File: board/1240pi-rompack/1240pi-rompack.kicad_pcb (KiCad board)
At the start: 4 copper layers, 73.7 x 50.8 mm, 5 parts, among them J1 HDMI_A, J2 HDMI_A, P1 CardEdge_ROMPACK

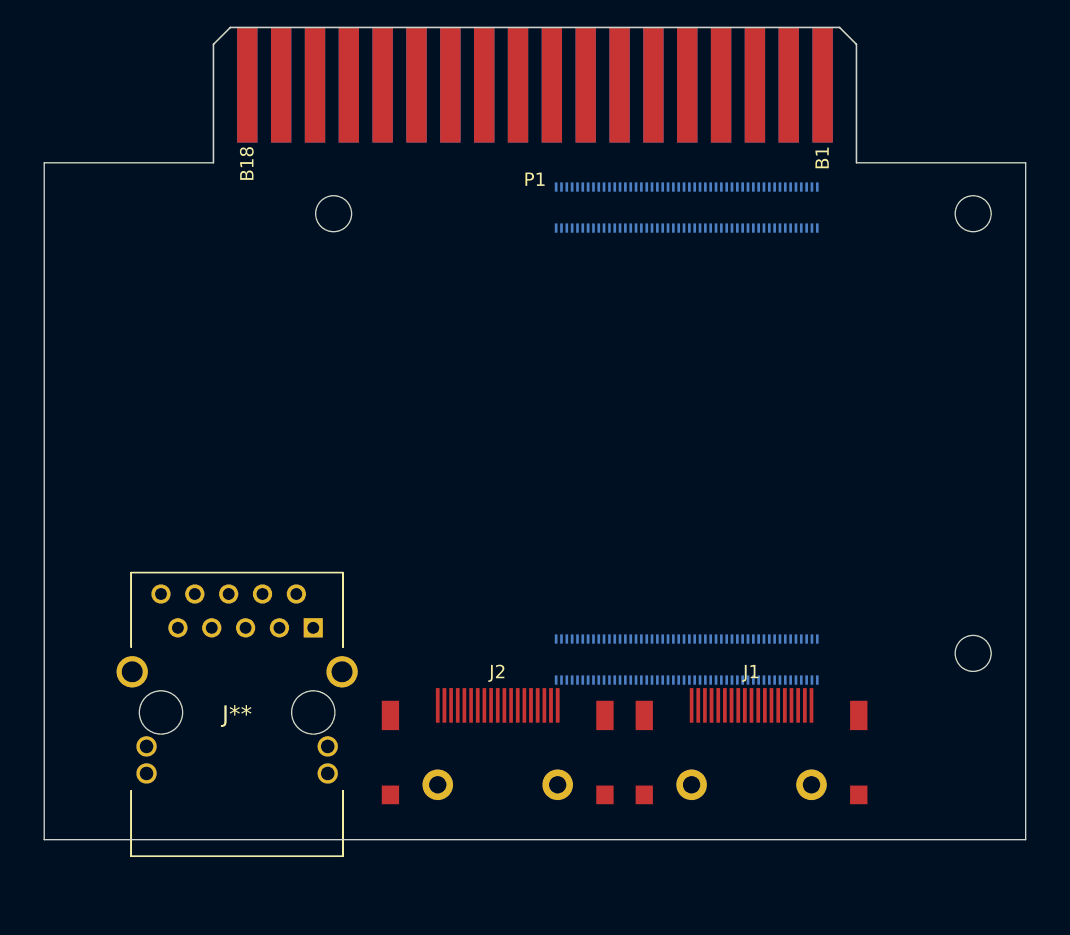
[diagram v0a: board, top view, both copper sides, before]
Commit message: Add more stuff to rompack board.
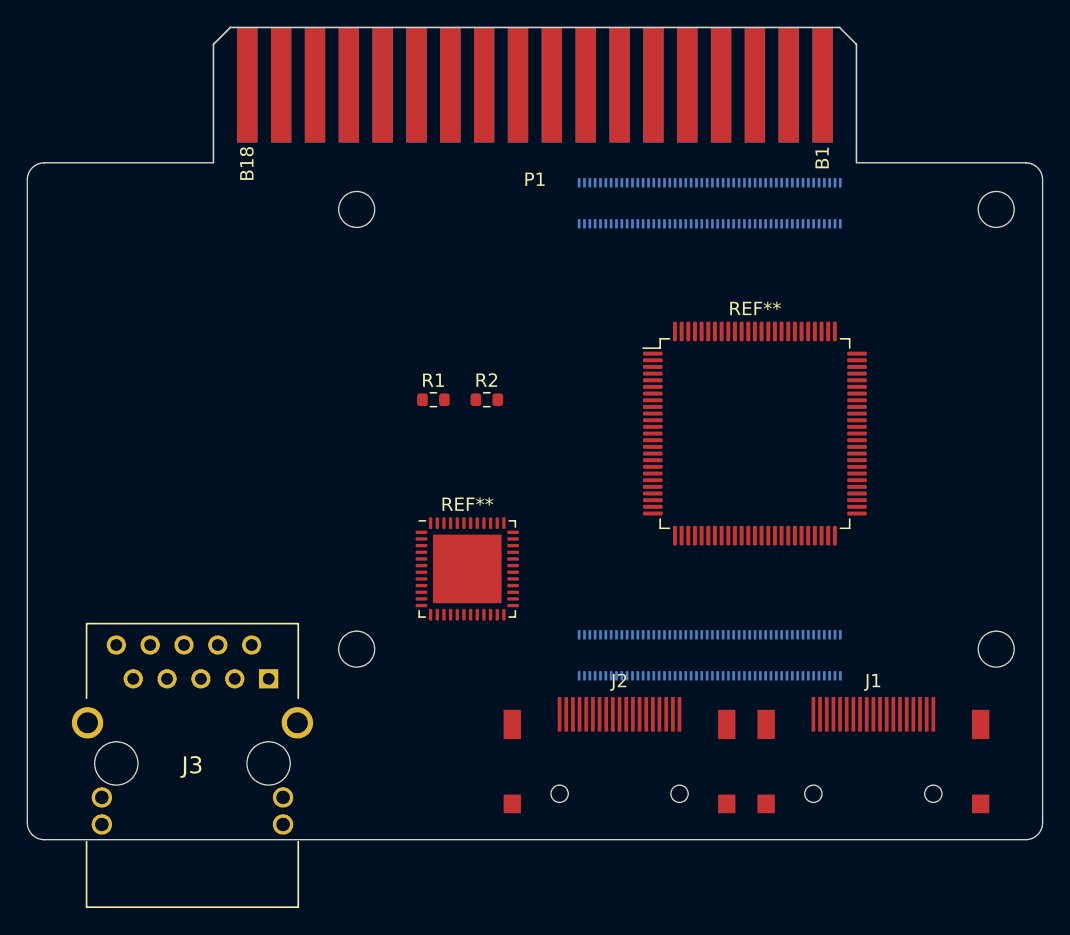
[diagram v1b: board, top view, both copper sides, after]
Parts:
- added R1: 470R, Resistor_SMD:R_0603_1608Metric, F.Cu at (144.8, 81.3)
- added R2: 470R, Resistor_SMD:R_0603_1608Metric, F.Cu at (148.8, 81.3)
- added REF**: QFN-48-1EP_7x7mm_P0.5mm_EP5.15x5.15mm, Package_DFN_QFN:QFN-48-1EP_7x7mm_P0.5mm_EP5.15x5.15mm, F.Cu at (147.3, 94.0)
- added REF**: VQFP-100_14x14mm_P0.5mm, Package_QFP:VQFP-100_14x14mm_P0.5mm, F.Cu at (168.9, 83.8)
- moved J1 9.17 mm to (177.8, 104.9)
- moved J2 9.17 mm to (158.8, 104.9)
- moved J3 5.09 mm to (132.4, 102.2)
- moved A1 1.76 mm to (187.0, 67.0)
- renumbered J** to J3
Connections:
- A1 pad 10: unconnected-(A1-Pad10) -> Net-(A1-Pad10)
- A1 pad 11: unconnected-(A1-Pad11) -> Net-(A1-Pad11)
- A1 pad 12: unconnected-(A1-Pad12) -> Net-(A1-Pad12)
- A1 pad 143: unconnected-(A1-Pad143) -> /HDMI/HDMI_OUT_HPD
- A1 pad 145: unconnected-(A1-Pad145) -> /HDMI/HDMI_OUT_SDA
- A1 pad 146: unconnected-(A1-Pad146) -> /HDMI/HDMI_OUT_D2_P
- A1 pad 147: unconnected-(A1-Pad147) -> /HDMI/HDMI_OUT_SCL
- A1 pad 148: unconnected-(A1-Pad148) -> /HDMI/HDMI_OUT_D2_N
- A1 pad 149: unconnected-(A1-Pad149) -> /HDMI/HDMI_OUT_CEC
- A1 pad 152: unconnected-(A1-Pad152) -> /HDMI/HDMI_OUT_D1_P
- A1 pad 154: unconnected-(A1-Pad154) -> /HDMI/HDMI_OUT_D1_N
- A1 pad 158: unconnected-(A1-Pad158) -> /HDMI/HDMI_OUT_D0_P
- A1 pad 160: unconnected-(A1-Pad160) -> /HDMI/HDMI_OUT_D0_N
- A1 pad 164: unconnected-(A1-Pad164) -> /HDMI/HDMI_OUT_CK_P
- A1 pad 166: unconnected-(A1-Pad166) -> /HDMI/HDMI_OUT_CK_N
- A1 pad 17: unconnected-(A1-Pad17) -> /CM4 Direct IO/ETH_LED_Y
- A1 pad 19: unconnected-(A1-Pad19) -> /CM4 Direct IO/ETH_LED_G
- A1 pad 3: unconnected-(A1-Pad3) -> Net-(A1-Pad3)
- A1 pad 4: unconnected-(A1-Pad4) -> Net-(A1-Pad4)
- A1 pad 5: unconnected-(A1-Pad5) -> Net-(A1-Pad5)
- A1 pad 6: unconnected-(A1-Pad6) -> Net-(A1-Pad6)
- A1 pad 9: unconnected-(A1-Pad9) -> Net-(A1-Pad9)
- J1 pad 1: unconnected-(J1-Pad1) -> /HDMI/HDMI_IN_D2_P
- J1 pad 10: unconnected-(J1-Pad10) -> /HDMI/HDMI_IN_CK_P
- J1 pad 12: unconnected-(J1-Pad12) -> /HDMI/HDMI_IN_CK_N
- J1 pad 13: unconnected-(J1-Pad13) -> /HDMI/HDMI_IN_CEC
- J1 pad 15: unconnected-(J1-Pad15) -> /HDMI/HDMI_IN_SCL
- J1 pad 16: unconnected-(J1-Pad16) -> /HDMI/HDMI_IN_SDA
- J1 pad 19: unconnected-(J1-Pad19) -> /HDMI/HDMI_IN_HPD
- J1 pad 3: unconnected-(J1-Pad3) -> /HDMI/HDMI_IN_D2_N
- J1 pad 4: unconnected-(J1-Pad4) -> /HDMI/HDMI_IN_D1_P
- J1 pad 6: unconnected-(J1-Pad6) -> /HDMI/HDMI_IN_D1_N
- J1 pad 7: unconnected-(J1-Pad7) -> /HDMI/HDMI_IN_D0_P
- J1 pad 9: unconnected-(J1-Pad9) -> /HDMI/HDMI_IN_D0_N
- J2 pad 1: unconnected-(J2-Pad1) -> /HDMI/HDMI_OUT_D2_P
- J2 pad 10: unconnected-(J2-Pad10) -> /HDMI/HDMI_OUT_CK_P
- J2 pad 12: unconnected-(J2-Pad12) -> /HDMI/HDMI_OUT_CK_N
- J2 pad 13: unconnected-(J2-Pad13) -> /HDMI/HDMI_OUT_CEC
- J2 pad 15: unconnected-(J2-Pad15) -> /HDMI/HDMI_OUT_SCL
- J2 pad 16: unconnected-(J2-Pad16) -> /HDMI/HDMI_OUT_SDA
- J2 pad 18: unconnected-(J2-Pad18) -> /HDMI/HDMI_OUT_+5V
- J2 pad 19: unconnected-(J2-Pad19) -> /HDMI/HDMI_OUT_HPD
- J2 pad 3: unconnected-(J2-Pad3) -> /HDMI/HDMI_OUT_D2_N
- J2 pad 4: unconnected-(J2-Pad4) -> /HDMI/HDMI_OUT_D1_P
- J2 pad 6: unconnected-(J2-Pad6) -> /HDMI/HDMI_OUT_D1_N
- J2 pad 7: unconnected-(J2-Pad7) -> /HDMI/HDMI_OUT_D0_P
- J2 pad 9: unconnected-(J2-Pad9) -> /HDMI/HDMI_OUT_D0_N
- J3 pad 1: (no net) -> Net-(A1-Pad12)
- J3 pad 10: (no net) -> Net-(A1-Pad5)
- J3 pad 2: (no net) -> Net-(A1-Pad10)
- J3 pad 3: (no net) -> Net-(A1-Pad4)
- J3 pad 4: (no net) -> Net-(A1-Pad6)
- J3 pad 5: (no net) -> unconnected-(J3-Pad5)
- J3 pad 6: (no net) -> unconnected-(J3-Pad5)
- J3 pad 7: (no net) -> Net-(A1-Pad11)
- J3 pad 8: (no net) -> Net-(A1-Pad9)
- J3 pad 9: (no net) -> Net-(A1-Pad3)
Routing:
- added copper zone on In1.Cu, net GND
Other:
- board size 73.7 x 50.8 mm -> 76.2 x 50.8 mm
- board text added: "Case opening clearance: top 600 mil, bottom 200 mil"
